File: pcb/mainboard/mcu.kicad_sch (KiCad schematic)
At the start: 30 parts, among them J6 Conn_01x08_MountingPin, SW1 SW, SW2 SW, U13 W25Q32JV, U14 RP2040, Y2 12MHz

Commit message: PCB r0p9
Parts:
- removed C100, C101, C156, C90, C91, C94, C95, C96, C97, C98, C99: 100nF, Capacitor_SMD:C_0402_1005Metric, symbol Device:C
- removed C102, C89: 1uF, Capacitor_SMD:C_0402_1005Metric, symbol Device:C
- removed C92, C93: 18pF, Capacitor_SMD:C_0402_1005Metric, symbol Device:C
- removed J6: Conn_01x08_MountingPin, Connector_FFC-FPC:Hirose_FH12-8S-0.5SH_1x08-1MP_P0.50mm_Horizontal, symbol Connector_Generic_MountingPin:Conn_01x08_MountingPin
- removed JP1: Jumper_2_Open, Jumper:SolderJumper-2_P1.3mm_Open_RoundedPad1.0x1.5mm, symbol Jumper:Jumper_2_Open
- removed R50, R51: 1M, Resistor_SMD:R_0402_1005Metric, symbol Device:R
- removed R57, R67: 1K/1%, Resistor_SMD:R_0402_1005Metric, symbol Device:R
- removed R58, R59: 27R, Resistor_SMD:R_0402_1005Metric, symbol Device:R
- removed R68, R69: 5.1K, Resistor_SMD:R_0402_1005Metric, symbol Device:R
- removed SW1, SW2: SW, Button_Switch_SMD:Panasonic_EVQPUL_EVQPUC, symbol Switch:SW_Push
- removed U13: W25Q32JV, Package_SON:WSON-8-1EP_6x5mm_P1.27mm_EP3.4x4.3mm, symbol Memory_Flash:W25Q32JVZP
- removed U14: RP2040, footprints:RP2040-QFN-56, symbol MCU_RaspberryPi:RP2040
- removed Y2: 12MHz, Crystal:Crystal_SMD_3225-4Pin_3.2x2.5mm, symbol Device:Crystal_GND24

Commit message: PCB r0p10 wip
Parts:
- added C214: 22uF, Capacitor_SMD:C_0603_1608Metric, symbol Device:C
- added C215: 100nF, Capacitor_SMD:C_0402_1005Metric, symbol Device:C
- added D19: LED GREEN, LED_SMD:LED_0603_1608Metric, symbol Device:LED
- added D20: LED RED, LED_SMD:LED_0603_1608Metric, symbol Device:LED
- added J7: MICRO_SD(TFC-WPAPR-08), footprints:TFC-WPAPR-08, symbol symbols:MICRO_SD(TFC-WPAPR-08)
- added R12, R14: 10K, Resistor_SMD:R_0402_1005Metric, symbol Device:R
- added R42, R43: 1K, Resistor_SMD:R_0402_1005Metric, symbol Device:R
- added SW1, SW2: SW, Button_Switch_SMD:Panasonic_EVQPUL_EVQPUC, symbol Switch:SW_Push
- added U14: STM32F407VGTx, Package_QFP:LQFP-100_14x14mm_P0.5mm, symbol MCU_ST_STM32F4:STM32F407VGTx
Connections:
- new net: D20.2 (A), R43.2
- new net: D19.2 (A), R42.2
- new net: U14.10 (VSS), U14.27 (VSS), U14.74 (VSS), U14.99 (VSS)
- new net +3V3: C214.1, C215.1, J7.4 (VDD), R12.1, R14.1
- new net EPD_VCOM_PWM: U14.67 (PA8)
- new net FL_PWM1: U14.42 (PE11)
- new net FL_PWM2: U14.44 (PE13)
- new net FPGA_CS: U14.77 (PA15)
- new net FPGA_MISO: U14.90 (PB4)
- new net FPGA_MOSI: U14.91 (PB5)
- new net FPGA_SCLK: U14.89 (PB3)
- new net FSMC_A16: U14.58 (PD11)
- new net FSMC_D0: U14.61 (PD14)
- new net FSMC_D1: U14.62 (PD15)
- new net FSMC_D2: U14.81 (PD0)
- new net FSMC_D3: U14.82 (PD1)
- new net FSMC_D4: U14.38 (PE7)
- new net FSMC_D5: U14.39 (PE8)
- new net FSMC_D6: U14.40 (PE9)
- new net FSMC_D7: U14.41 (PE10)
- new net FSMC_NE1: U14.88 (PD7)
- new net FSMC_NOE: U14.85 (PD4)
- new net FSMC_NWE: U14.86 (PD5)
- new net GND: C214.2, C215.2, D19.1 (K), D20.1 (K), J7.10, J7.11, J7.12, J7.13, J7.6 (VSS), SW1.2, SW2.2
- new net G_LED: R42.1
- new net I2C1_SCL: R14.2, U14.92 (PB6)
- new net I2C1_SDA: R12.2, U14.93 (PB7)
- new net KEY1: SW2.1
- new net KEY2: SW1.1
- new net MCU_SWCLK: U14.76 (PA14)
- new net MCU_SWDIO: U14.72 (PA13)
- new net R_LED: R43.1
- new net SDIO_CLK: J7.5 (CLK/SCLK), U14.80 (PC12)
- new net SDIO_CMD: J7.3 (CMD/DI), U14.83 (PD2)
- new net SDIO_DAT0: J7.7 (DAT0/DO), U14.65 (PC8)
- new net SDIO_DAT1: J7.8 (DAT1/RES), U14.66 (PC9)
- new net SDIO_DAT2: J7.1 (DAT2/RES), U14.78 (PC10)
- new net SDIO_DAT3: J7.2 (CD/DAT3/CS), U14.79 (PC11)
- new net USB_DN: U14.70 (PA11)
- new net USB_DP: U14.71 (PA12)
- new net VBUS_MEA: U14.36 (PB1)
- new net VCOM_MEA: U14.35 (PB0)
- new net VGH_MEA: U14.26 (PA3)
- new net VGL_MEA: U14.32 (PA7)
- new net VN1_MEA: U14.29 (PA4)
- new net VN2_MEA: U14.30 (PA5)
- new net VN3_MEA: U14.31 (PA6)
- new net VP1_MEA: U14.23 (PA0)
- new net VP2_MEA: U14.24 (PA1)
- new net VP3_MEA: U14.25 (PA2)
- no-connect marks 0 -> 2

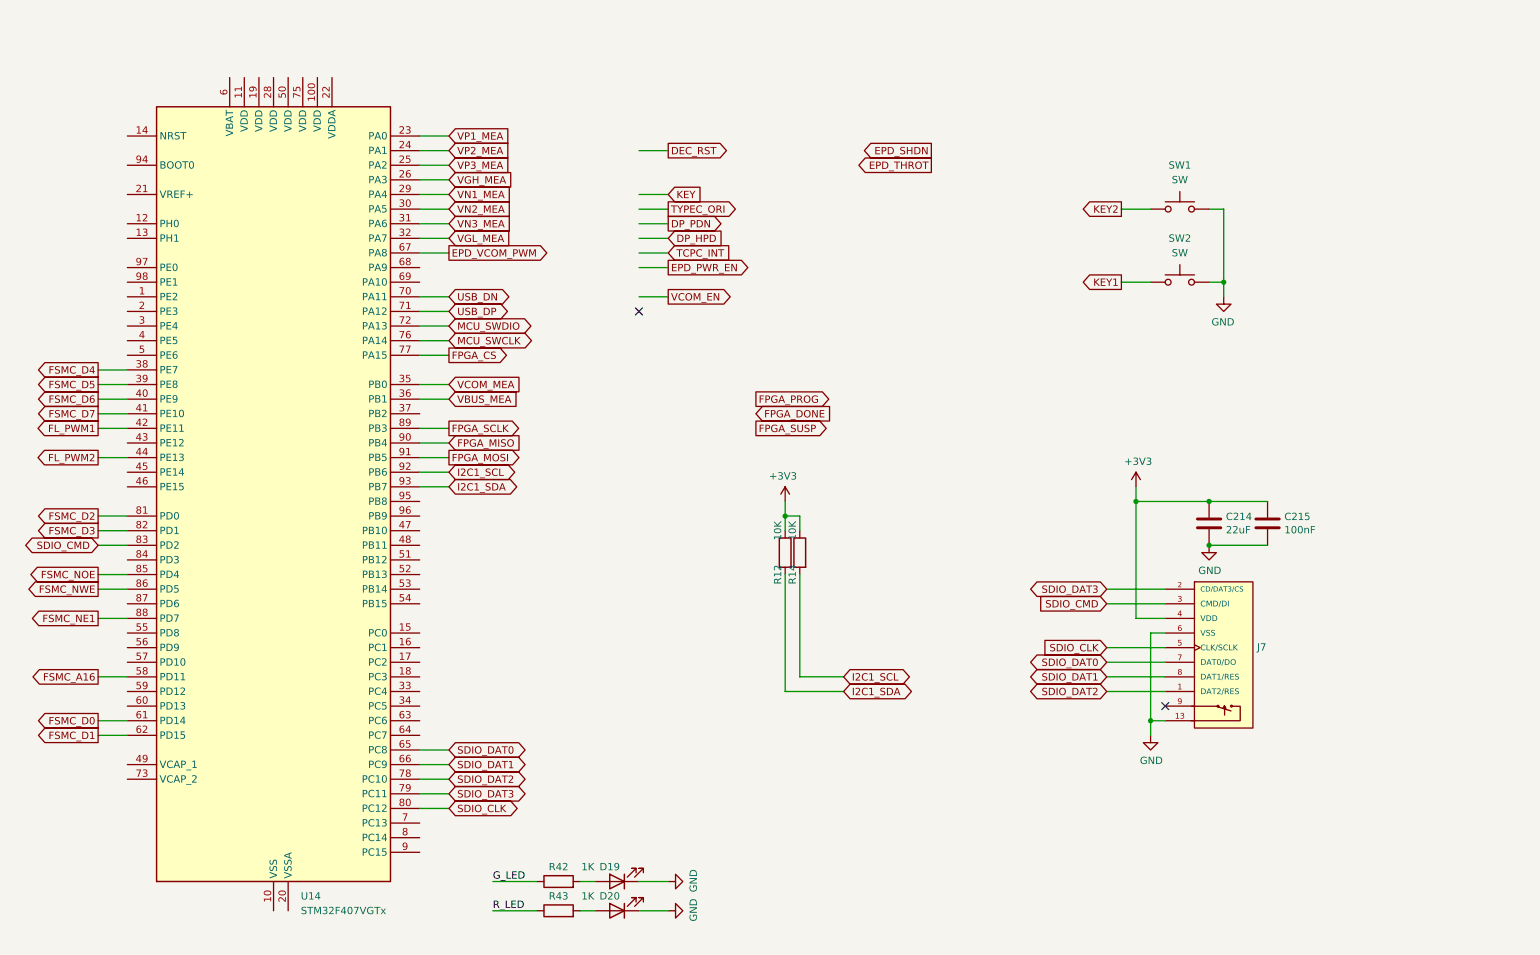
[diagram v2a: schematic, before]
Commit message: PCB r0p10
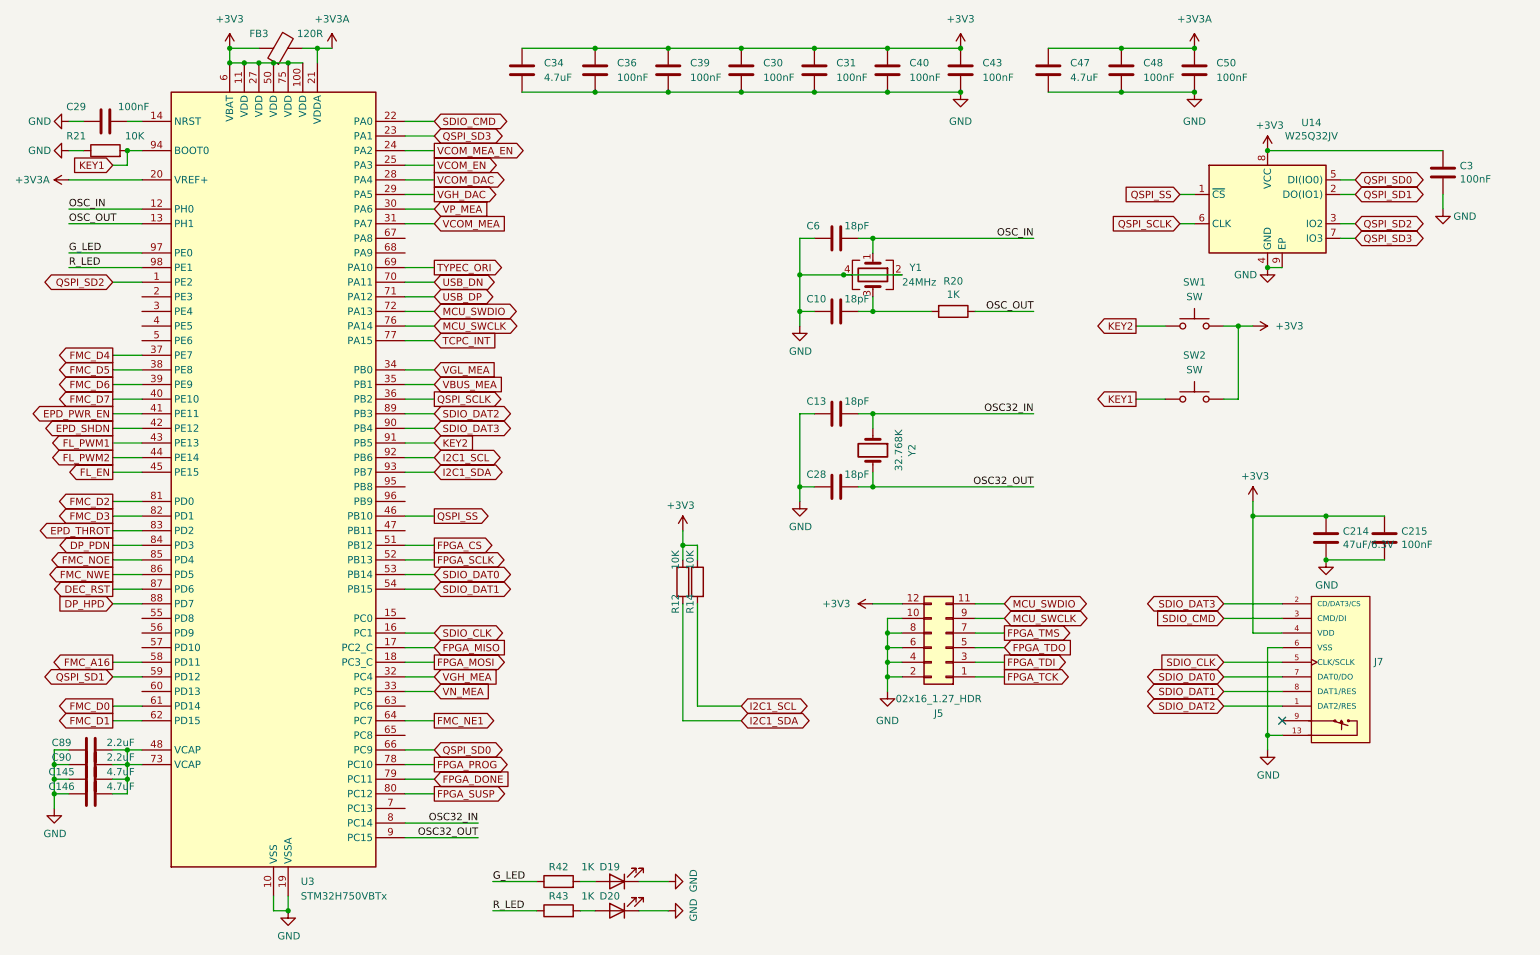
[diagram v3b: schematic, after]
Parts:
- removed U14: STM32F407VGTx, Package_QFP:LQFP-100_14x14mm_P0.5mm, symbol MCU_ST_STM32F4:STM32F407VGTx
- added C10, C13, C28, C6: 18pF, Capacitor_SMD:C_0402_1005Metric, symbol Device:C
- added C145, C146, C34, C47: 4.7uF, Capacitor_SMD:C_0402_1005Metric, symbol Device:C
- added C29, C3, C30, C31, C36, C39, C40, C43, C48, C50: 100nF, Capacitor_SMD:C_0402_1005Metric, symbol Device:C
- added C89, C90: 2.2uF, Capacitor_SMD:C_0402_1005Metric, symbol Device:C
- added FB3: 120R, Inductor_SMD:L_0603_1608Metric, symbol Device:FerriteBead
- added J5: 02x16_1.27_HDR, Connector_PinSocket_1.27mm:PinSocket_2x06_P1.27mm_Vertical_SMD, symbol Connector_Generic:Conn_02x06_Odd_Even
- added R20: 1K, Resistor_SMD:R_0402_1005Metric, symbol Device:R
- added R21: 10K, Resistor_SMD:R_0402_1005Metric, symbol Device:R
- added U14: W25Q32JV, Package_SON:WSON-8-1EP_6x5mm_P1.27mm_EP3.4x4.3mm, symbol Memory_Flash:W25Q32JVZP
- added U3: STM32H750VBTx, Package_QFP:LQFP-100_14x14mm_P0.5mm, symbol MCU_ST_STM32H7:STM32H750VBTx
- added Y1: 24MHz, Crystal:Crystal_SMD_3225-4Pin_3.2x2.5mm, symbol Device:Crystal_GND24
- added Y2: 32.768K, Crystal:Crystal_SMD_TXC_9HT11-2Pin_2.0x1.2mm_HandSoldering, symbol Device:Crystal
- C214: value 22uF -> 47uF/6.3V
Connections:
- net +3V3: now also SW1.2, SW2.2, C3.1, C30.1, C31.1, C34.1, C36.1, C39.1, C40.1, C43.1, FB3.1, J5.12 (Pin_12), U14.8 (VCC), U3.100 (VDD), U3.11 (VDD), U3.27 (VDD), U3.50 (VDD), U3.6 (VBAT), U3.75 (VDD)
- net DEC_RST: now also U3.87 (PD6)
- net DP_HPD: now also U3.88 (PD7)
- net DP_PDN: now also U3.84 (PD3)
- net EPD_PWR_EN: now also U3.41 (PE11)
- net EPD_SHDN: now also U3.42 (PE12)
- net EPD_THROT: now also U3.83 (PD2)
- net FL_PWM1: now also U3.43 (PE13)
- net FL_PWM2: now also U3.44 (PE14)
- net FPGA_CS: now also U3.51 (PB12)
- net FPGA_DONE: now also U3.79 (PC11)
- net FPGA_MISO: now also U3.17 (PC2_C)
- net FPGA_MOSI: now also U3.18 (PC3_C)
- net FPGA_PROG: now also U3.78 (PC10)
- net FPGA_SCLK: now also U3.52 (PB13)
- net FPGA_SUSP: now also U3.80 (PC12)
- net GND: now also C10.2, C13.2, C145.1, C146.1, C28.2, C29.1, C3.2, C30.2, C31.2, C34.2, C36.2, C39.2, C40.2, C43.2, C47.2, C48.2, C50.2, C6.2, C89.1, C90.1, J5.10 (Pin_10), J5.2 (Pin_2), J5.4 (Pin_4), J5.6 (Pin_6), J5.8 (Pin_8), R21.1, U14.4 (GND), U14.9 (EP), U3.10 (VSS), U3.19 (VSSA), U3.26 (VSS), U3.49 (VSS), U3.74 (VSS), U3.99 (VSS), Y1.2, Y1.4; no longer SW1.2, SW2.2
- net G_LED: now also U3.97 (PE0)
- net I2C1_SCL: now also U3.92 (PB6)
- net I2C1_SDA: now also U3.93 (PB7)
- net KEY1: now also R21.2, U3.94 (BOOT0)
- net KEY2: now also U3.91 (PB5)
- net MCU_SWCLK: now also J5.9 (Pin_9), U3.76 (PA14)
- net MCU_SWDIO: now also J5.11 (Pin_11), U3.72 (PA13)
- net R_LED: now also U3.98 (PE1)
- net SDIO_CLK: now also U3.16 (PC1)
- net SDIO_CMD: now also U3.22 (PA0)
- net SDIO_DAT0: now also U3.53 (PB14)
- net SDIO_DAT1: now also U3.54 (PB15)
- net SDIO_DAT2: now also U3.89 (PB3)
- net SDIO_DAT3: now also U3.90 (PB4)
- net TCPC_INT: now also U3.77 (PA15)
- net TYPEC_ORI: now also U3.69 (PA10)
- net USB_DN: now also U3.70 (PA11)
- net USB_DP: now also U3.71 (PA12)
- net VBUS_MEA: now also U3.35 (PB1)
- net VCOM_EN: now also U3.25 (PA3)
- net VCOM_MEA: now also U3.31 (PA7)
- net VGH_MEA: now also U3.32 (PC4)
- net VGL_MEA: now also U3.34 (PB0)
- new net: C145.2, C146.2, C89.2, C90.2, U3.48 (VCAP), U3.73 (VCAP)
- new net: C10.1, R20.2, Y1.3
- new net: C29.2, U3.14 (NRST)
- new net +3V3A: C47.1, C48.1, C50.1, FB3.2, U3.20 (VREF+), U3.21 (VDDA)
- new net FL_EN: U3.45 (PE15)
- new net FMC_A16: U3.58 (PD11)
- new net FMC_D0: U3.61 (PD14)
- new net FMC_D1: U3.62 (PD15)
- new net FMC_D2: U3.81 (PD0)
- new net FMC_D3: U3.82 (PD1)
- new net FMC_D4: U3.37 (PE7)
- new net FMC_D5: U3.38 (PE8)
- new net FMC_D6: U3.39 (PE9)
- new net FMC_D7: U3.40 (PE10)
- new net FMC_NE1: U3.64 (PC7)
- new net FMC_NOE: U3.85 (PD4)
- new net FMC_NWE: U3.86 (PD5)
- new net FPGA_TCK: J5.1 (Pin_1)
- new net FPGA_TDI: J5.3 (Pin_3)
- new net FPGA_TDO: J5.5 (Pin_5)
- new net FPGA_TMS: J5.7 (Pin_7)
- new net OSC32_IN: C13.1, U3.8 (PC14), Y2.1
- new net OSC32_OUT: C28.1, U3.9 (PC15), Y2.2
- new net OSC_IN: C6.1, U3.12 (PH0), Y1.1
- new net OSC_OUT: R20.1, U3.13 (PH1)
- new net QSPI_SCLK: U14.6 (CLK), U3.36 (PB2)
- new net QSPI_SD0: U14.5 (DI(IO0)), U3.66 (PC9)
- new net QSPI_SD1: U14.2 (DO(IO1)), U3.59 (PD12)
- new net QSPI_SD2: U14.3 (IO2), U3.1 (PE2)
- new net QSPI_SD3: U14.7 (IO3), U3.23 (PA1)
- new net QSPI_SS: U14.1 (~{CS}), U3.46 (PB10)
- new net VCOM_DAC: U3.28 (PA4)
- new net VCOM_MEA_EN: U3.24 (PA2)
- new net VGH_DAC: U3.29 (PA5)
- new net VN_MEA: U3.33 (PC5)
- new net VP_MEA: U3.30 (PA6)
- no-connect marks 2 -> 1
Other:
- moved on the sheet: C214, C215, J7, R12, R14, SW1, SW2

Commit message: PCB r0p13
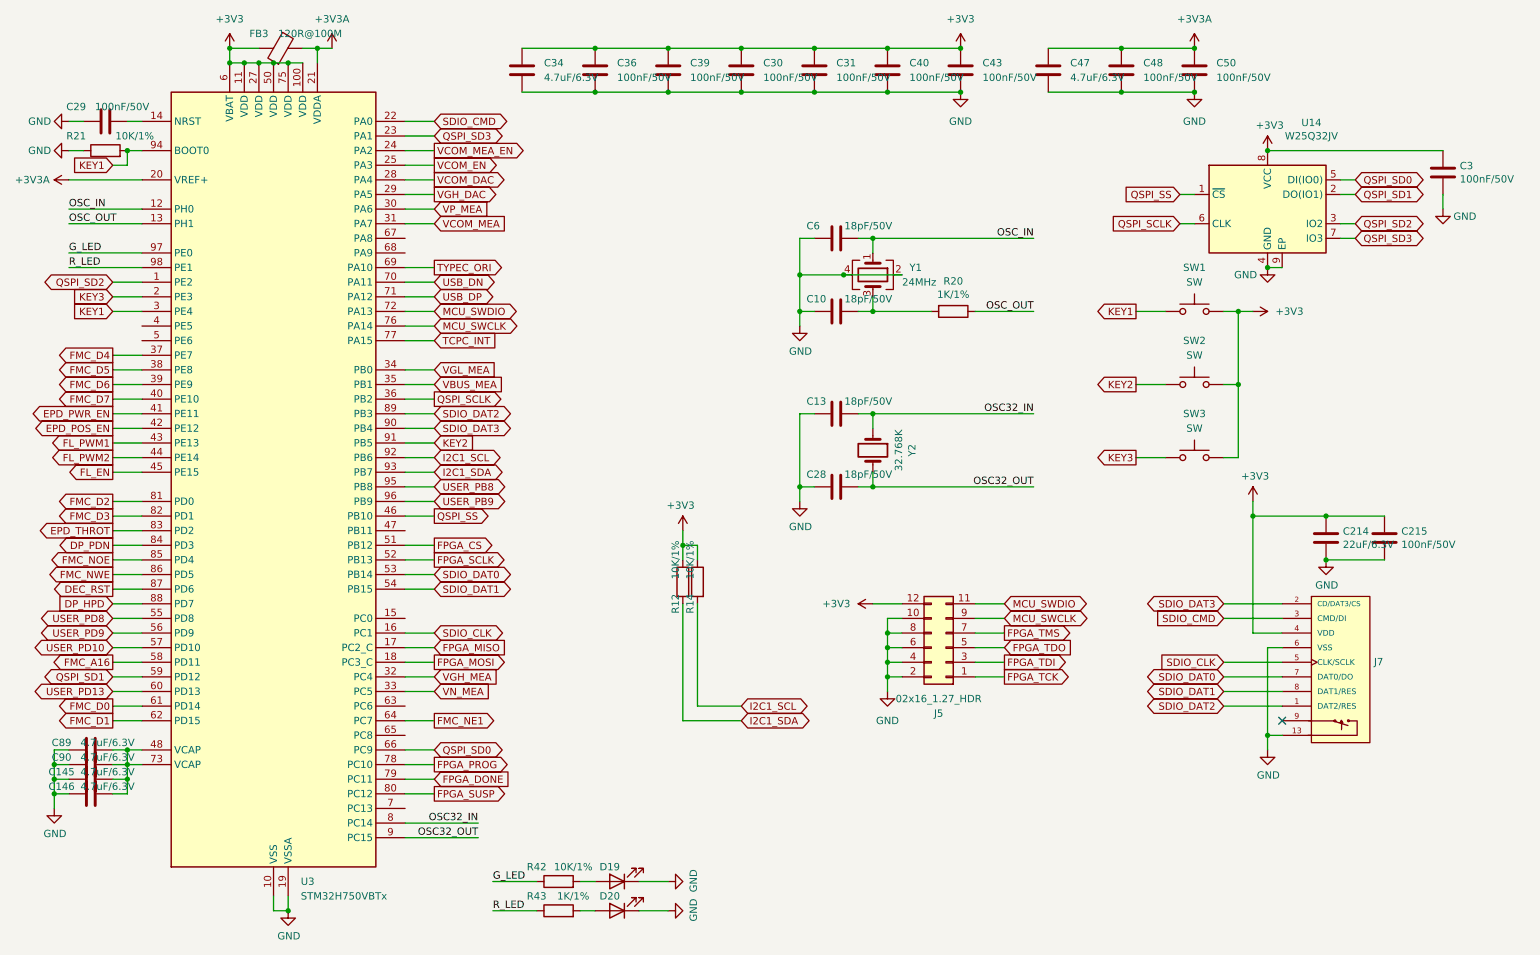
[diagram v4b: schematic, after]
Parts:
- added SW3: SW, Button_Switch_SMD:Panasonic_EVQPUL_EVQPUC, symbol Switch:SW_Push
- C10, C13, C28, C6: value 18pF -> 18pF/50V
- C145, C146, C34, C47: value 4.7uF -> 4.7uF/6.3V
- C214: value 47uF/6.3V -> 22uF/6.3V
- C215, C29, C3, C30, C31, C36, C39, C40, C43, C48, C50: value 100nF -> 100nF/50V
- C89, C90: value 2.2uF -> 4.7uF/6.3V
- FB3: value 120R -> 120R@100M
- R12, R14, R21: value 10K -> 10K/1%
- R20, R43: value 1K -> 1K/1%
- R42: value 1K -> 10K/1%
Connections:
- net +3V3: now also SW3.2
- net KEY1: now also SW1.1, U3.3 (PE4); no longer SW2.1
- net KEY2: now also SW2.1; no longer SW1.1
- net KEY3: now reaches U3.2 (PE3)
- net KEY3: now also SW3.1
- net USER_PD8: now reaches U3.55 (PD8)
- net USER_PD9: now reaches U3.56 (PD9)
- net USER_PD10: now reaches U3.57 (PD10)
- net USER_PD13: now reaches U3.60 (PD13)
- net USER_PB8: now reaches U3.95 (PB8)
- net USER_PB9: now reaches U3.96 (PB9)
- net EPD_SHDN renamed EPD_POS_EN
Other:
- company: Copyright 2024 Wenting Zhang -> Copyright 2025 Wenting Zhang
- moved on the sheet: SW1, SW2
